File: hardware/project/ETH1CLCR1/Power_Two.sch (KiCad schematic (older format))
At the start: 53 parts, among them U1501 LT8330_S6, U1502 LT8330_S6, U1503 MC7815BD2TG, U1504 MC7915BD2TG, U1505 MC78M12ABDTRKG, U1506 MC79M12CDTG, U1507 TSR2-2450, U1508 TSR1-2490, U1509 LM1117IMP-3.3/NOPB, U1510 LM1117IMP-3.3/NOPB, U1511 LM1117IMP-5.0/NOPB

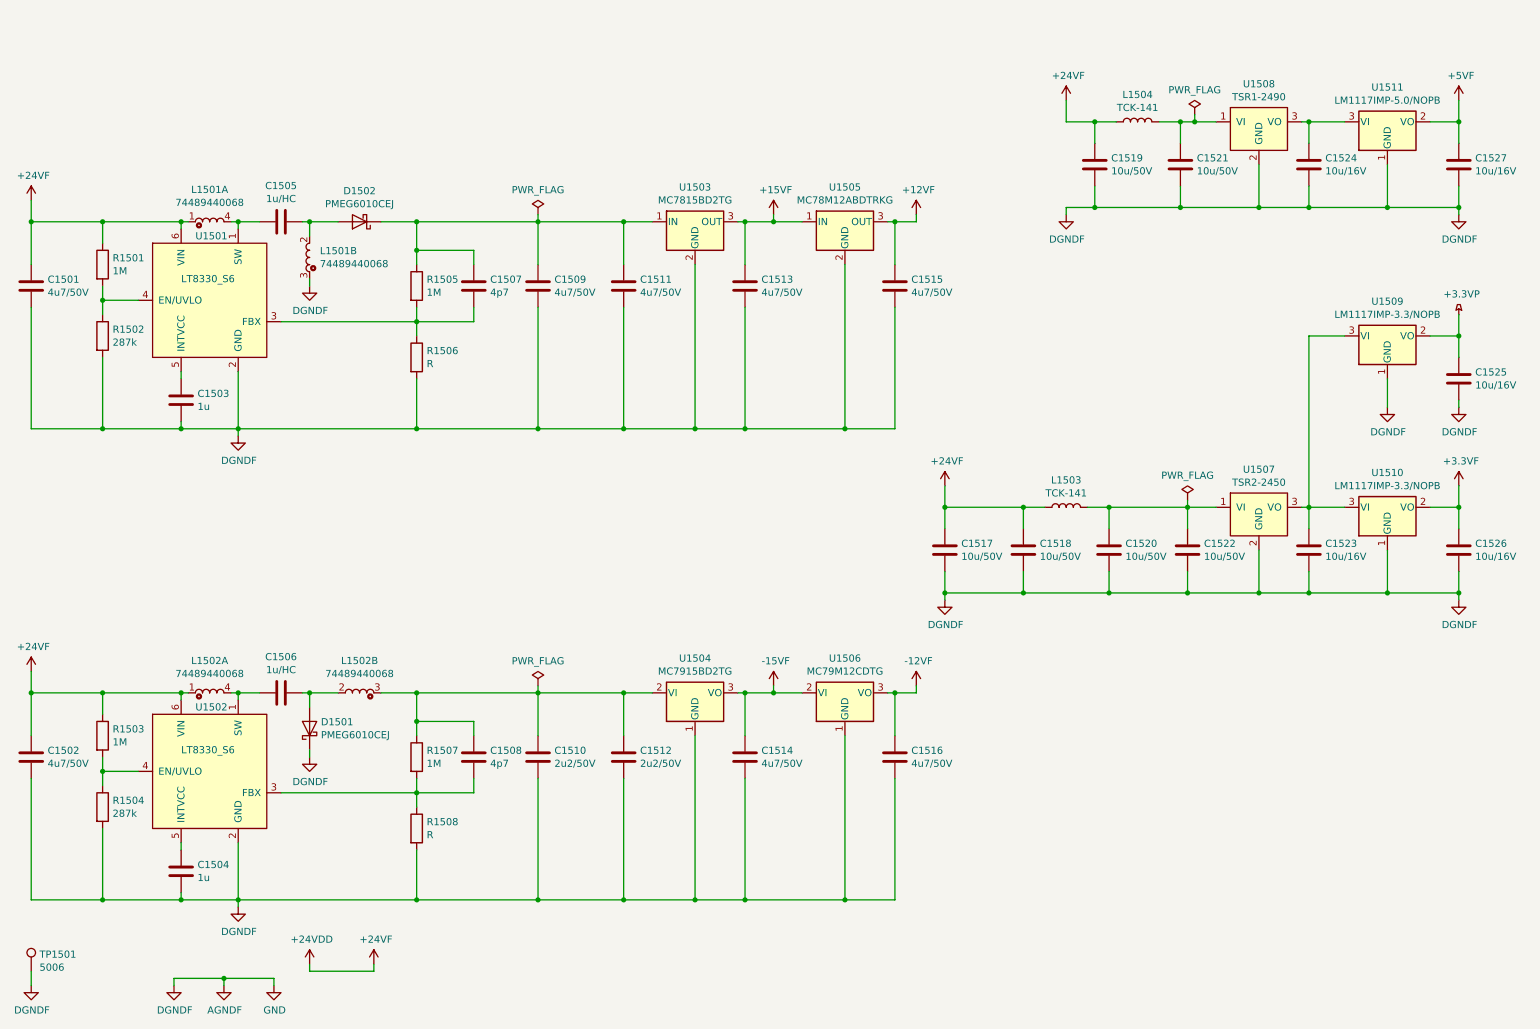
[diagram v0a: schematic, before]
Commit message: PCB layout
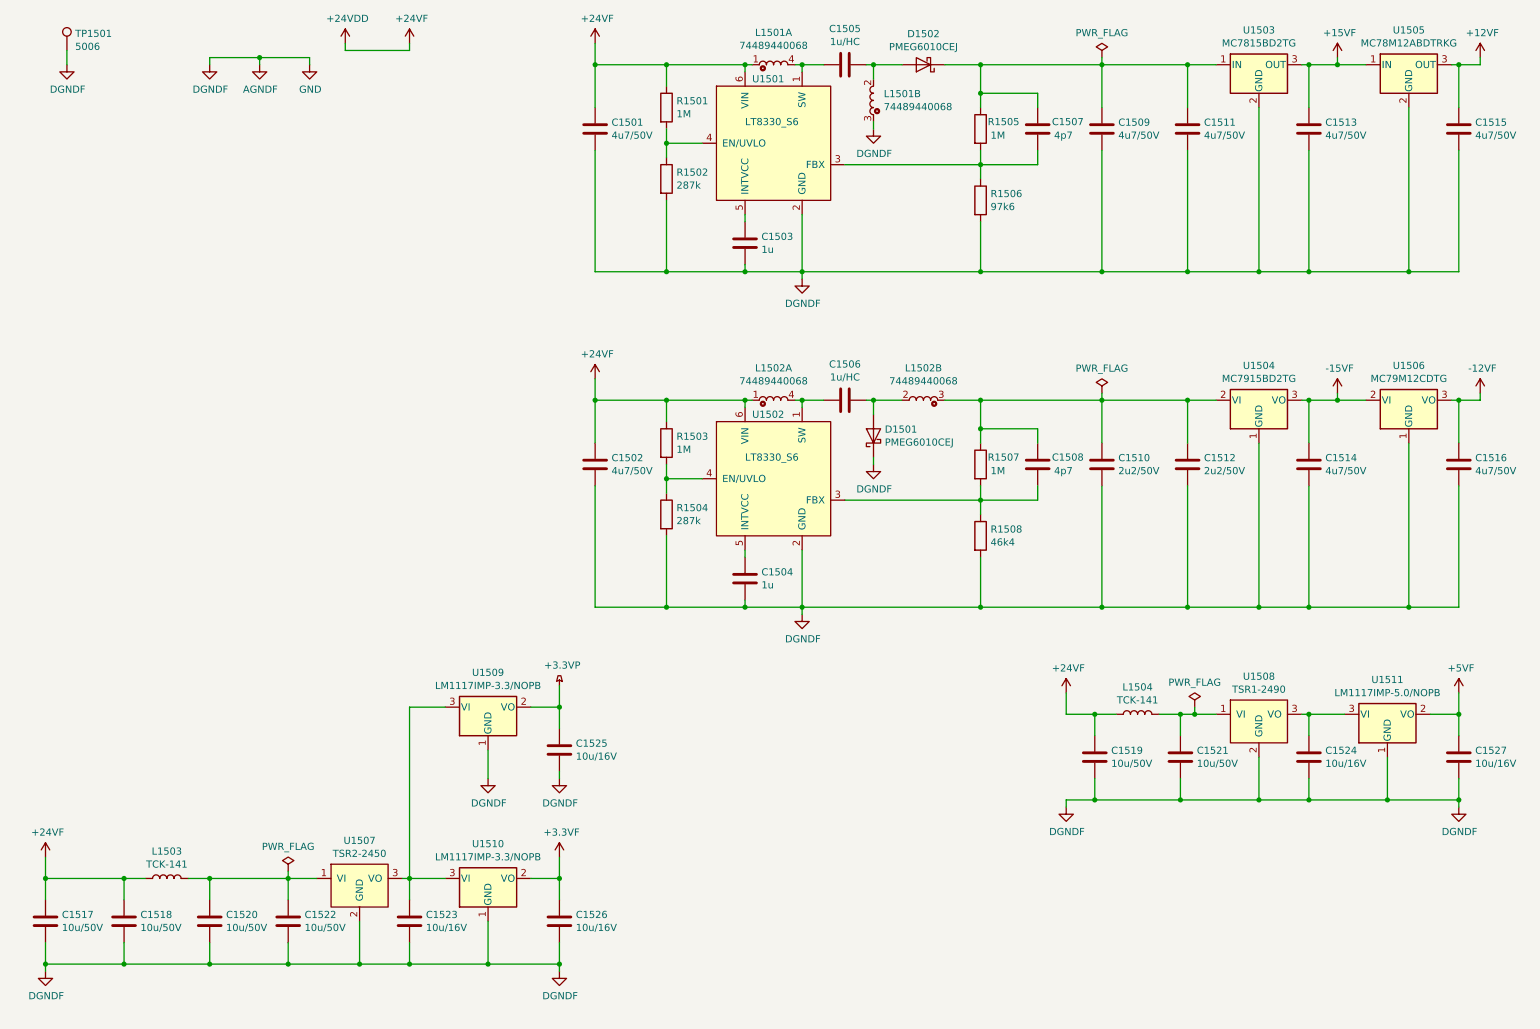
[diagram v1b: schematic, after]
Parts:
- R1506: value R -> 97k6
- R1508: value R -> 46k4
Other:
- moved on the sheet: C1501, C1502, C1503, C1504, C1505, C1506, C1507, C1508, C1509, C1510, C1511, C1512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
